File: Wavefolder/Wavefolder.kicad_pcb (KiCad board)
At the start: 2 copper layers, 25 x 200 mm, 39 parts, among them J1 Sig1, J2 EuroPower, J3 Sig2, J4 Out1, J5 Out2, J6 CV2, Q1 BC547, Q2 BC557, Q3 BC557, Q4 BC547, Q5 BC557, Q6 BC547, U1 TL074, U2 TL082, U3 TL074

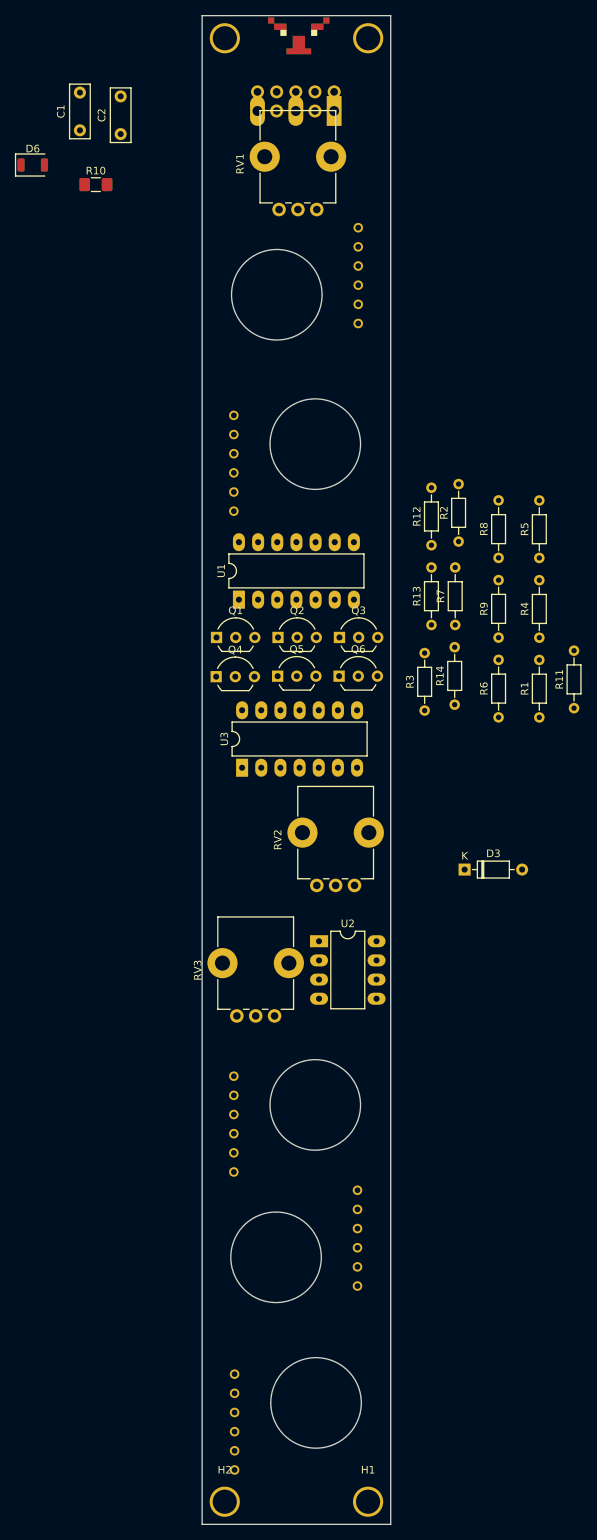
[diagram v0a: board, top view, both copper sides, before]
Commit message: Wavefolder layout
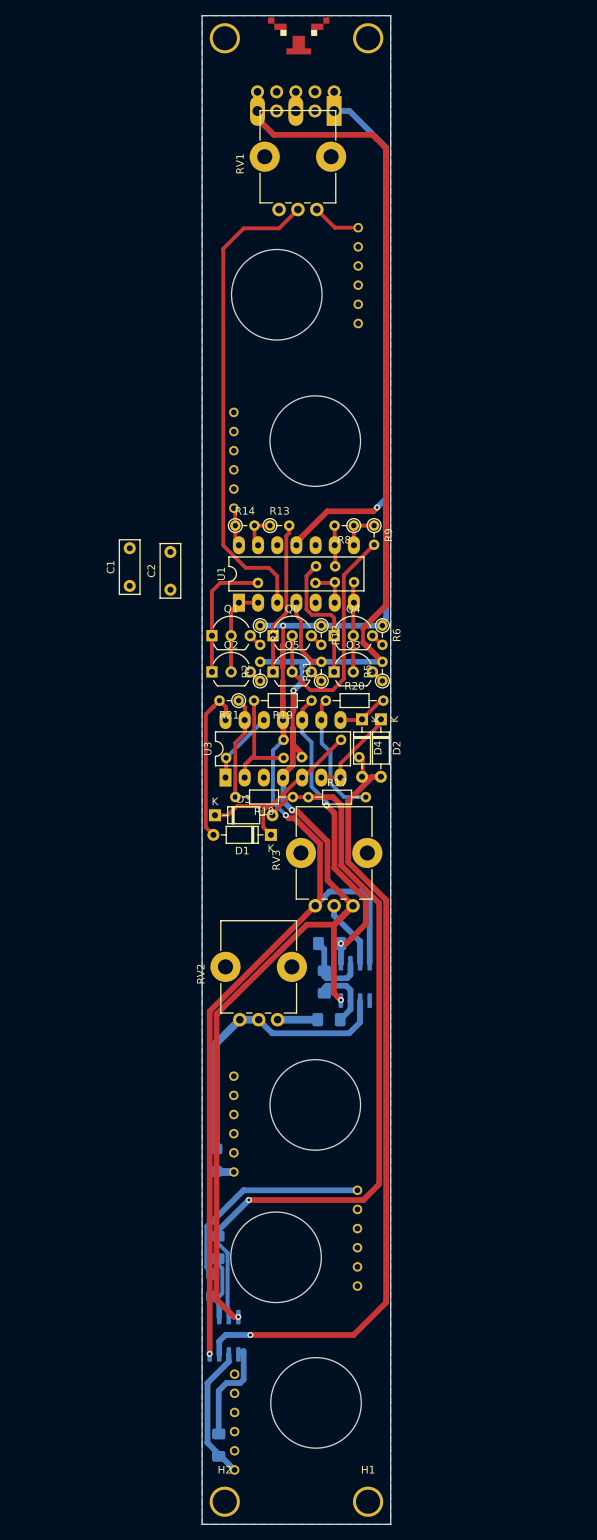
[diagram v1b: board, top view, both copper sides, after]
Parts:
- removed D6: LED, LED_SMD:LED_1206_3216Metric_ReverseMount_Hole1.8x2.4mm
- removed R10: 1k, Resistor_SMD:R_1206_3216Metric_Pad1.42x1.75mm_HandSolder
- added D1: 1N4148, Diode_THT:D_DO-35_SOD27_P7.62mm_Horizontal, F.Cu at (21.1, 120.6)
- added D2: 1N4148, Diode_THT:D_DO-35_SOD27_P7.62mm_Horizontal, F.Cu at (35.7, 105.3)
- added D4: 1N4148, Diode_THT:D_DO-35_SOD27_P7.62mm_Horizontal, F.Cu at (33.2, 105.3)
- added R15: 100k, Resistor_SMD:R_1206_3216Metric_Pad1.42x1.75mm_HandSolder, B.Cu at (13.4, 180.3)
- added R16: 100k, Resistor_SMD:R_1206_3216Metric_Pad1.42x1.75mm_HandSolder, B.Cu at (14.1, 175.3)
- added R17: 100k, Resistor_THT:R_Axial_DIN0204_L3.6mm_D1.6mm_P7.62mm_Horizontal, F.Cu at (26.1, 115.6)
- added R18: 100k, Resistor_THT:R_Axial_DIN0204_L3.6mm_D1.6mm_P7.62mm_Horizontal, F.Cu at (24.0, 115.6)
- added R19: 100k, Resistor_THT:R_Axial_DIN0204_L3.6mm_D1.6mm_P7.62mm_Horizontal, F.Cu at (26.5, 102.8)
- added R20: 100k, Resistor_THT:R_Axial_DIN0204_L3.6mm_D1.6mm_P7.62mm_Horizontal, F.Cu at (28.4, 102.8)
- added R21: 100k, Resistor_THT:R_Axial_DIN0204_L3.6mm_D1.6mm_P2.54mm_Vertical, F.Cu at (16.8, 102.8)
- added R22: 100k, Resistor_THT:R_Axial_DIN0204_L3.6mm_D1.6mm_P7.62mm_Horizontal, B.Cu at (22.8, 110.4)
- added R23: 15k, Resistor_THT:R_Axial_DIN0204_L3.6mm_D1.6mm_P7.62mm_Horizontal, B.Cu at (22.8, 108.0)
- added R24: 15k, Resistor_THT:R_Axial_DIN0204_L3.6mm_D1.6mm_P7.62mm_Horizontal, B.Cu at (32.8, 110.3)
- added R25: 1k, Resistor_SMD:R_1206_3216Metric_Pad1.42x1.75mm_HandSolder, B.Cu at (14.2, 201.5)
- added R26: 100k, Resistor_SMD:R_1206_3216Metric_Pad1.42x1.75mm_HandSolder, B.Cu at (13.8, 163.7)
- added R27: 100k, Resistor_SMD:R_1206_3216Metric_Pad1.42x1.75mm_HandSolder, B.Cu at (28.8, 145.1)
- added R28: 100k, Resistor_SMD:R_1206_3216Metric_Pad1.42x1.75mm_HandSolder, B.Cu at (28.2, 140.1)
- added R29: 100k, Resistor_SMD:R_1206_3216Metric_Pad1.42x1.75mm_HandSolder, B.Cu at (28.9, 135.0)
- added U4: TL082, Package_SO:SOIC-8_3.9x4.9mm_P1.27mm, B.Cu at (14.9, 187.0)
- R1, R11, R12, R13, R14, R2, R5, R6, R8, R9: footprint Resistor_THT:R_Axial_DIN0204_L3.6mm_D1.6mm_P7.62mm_Horizontal -> Resistor_THT:R_Axial_DIN0204_L3.6mm_D1.6mm_P2.54mm_Vertical
- R3: moved to B.Cu
- R4, R7: footprint Resistor_THT:R_Axial_DIN0204_L3.6mm_D1.6mm_P7.62mm_Horizontal -> Resistor_THT:R_Axial_DIN0204_L3.6mm_D1.6mm_P2.54mm_Vertical; moved to B.Cu
- U2: footprint Package_DIP:DIP-8_W7.62mm_LongPads -> Package_SO:SOIC-8_3.9x4.9mm_P1.27mm; moved to B.Cu
- moved C1 60.8 mm to (2.40, 87.6)
- moved C2 60.8 mm to (7.80, 88.1)
- moved R1 39.0 mm to (19.7, 92.9), turned to 270 degrees
- moved R14 37.5 mm to (16.4, 79.6), turned to 0 degrees
- moved D3 33.9 mm to (13.7, 118.0)
- moved R11 33.7 mm to (27.8, 100.2)
- moved R2 32.1 mm to (19.7, 100.2)
- moved R4 28.1 mm to (29.6, 87.1), turned to 0 degrees
- moved R3 27.8 mm to (19.4, 87.2), turned to 0 degrees
- moved R5 26.4 mm to (35.9, 100.2)
- moved R13 25.1 mm to (21.0, 79.6), turned to 0 degrees
- moved R9 22.2 mm to (34.8, 79.6), turned to 270 degrees
- moved RV2 20.5 mm to (22.0, 145.1)
- moved R7 20.0 mm to (27.1, 85.0), turned to 0 degrees
- moved R8 19.7 mm to (32.1, 79.6), turned to 180 degrees
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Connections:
- D3 pad 1: Net-(D3-Pad1) -> Net-(D1-Pad1)
- D3 pad 2: Net-(D3-Pad2) -> /~Sig2
- R13 pad 1: Net-(Q5-Pad1) -> Net-(R13-Pad1)
- R13 pad 2: Net-(R13-Pad2) -> Net-(Q5-Pad1)
- R14 pad 1: Net-(R13-Pad2) -> /Out1
- R14 pad 2: /Out1 -> Net-(R13-Pad1)
- R8 pad 1: Net-(R7-Pad2) -> Net-(R8-Pad1)
- R8 pad 2: Net-(R8-Pad2) -> Net-(R7-Pad2)
- R9 pad 1: Net-(R8-Pad2) -> Net-(R8-Pad1)
- RV2 pad 2: Net-(RV2-Pad2) -> Net-(R26-Pad2)
- RV2 pad 3: Net-(RV2-Pad3) -> Net-(R26-Pad2)
- RV3 pad 1: Net-(RV3-Pad1) -> +12V
- RV3 pad 3: Net-(RV3-Pad3) -> -12V
- U1 pad 1: (no net) -> Net-(Q1-Pad2)
- U1 pad 13: Net-(R13-Pad2) -> Net-(R13-Pad1)
- U1 pad 2: (no net) -> Net-(Q1-Pad2)
- U1 pad 3: (no net) -> Net-(RV1-Pad2)
- U1 pad 8: Net-(R8-Pad2) -> Net-(R8-Pad1)
- U2 pad 1: Net-(U2-Pad1) -> /Offset
- U2 pad 3: Net-(U2-Pad3) -> Net-(RV3-Pad2)
- U2 pad 5: Net-(U2-Pad5) -> GND
- U2 pad 6: Net-(U2-Pad6) -> Net-(R26-Pad2)
- U3 pad 1: (no net) -> /~Offset
- U3 pad 10: (no net) -> /Offset
- U3 pad 11: (no net) -> -12V
- U3 pad 12: (no net) -> /~Offset
- U3 pad 13: (no net) -> Net-(R18-Pad2)
- U3 pad 14: (no net) -> /Bottom
- U3 pad 2: (no net) -> Net-(R19-Pad2)
- U3 pad 3: (no net) -> GND
- U3 pad 4: (no net) -> +12V
- U3 pad 5: Net-(U3-Pad5) -> Net-(D1-Pad1)
- U3 pad 6: Net-(U3-Pad6) -> Net-(D2-Pad1)
- U3 pad 7: Net-(U3-Pad7) -> Net-(D2-Pad1)
- U3 pad 8: (no net) -> /Top
- U3 pad 9: (no net) -> Net-(R17-Pad2)
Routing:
- net +12V: track 0.00 -> 247.2 mm, vias 0 -> 4
- net -12V: track 0.00 -> 229.7 mm, vias 0 -> 4
- net /Out2: track 0.00 -> 105.4 mm, vias 0 -> 1
- net /~Sig2: track 0.00 -> 98.9 mm, vias 0 -> 1
- net Net-(RV1-Pad2): track 0.00 -> 63.7 mm
- net /Offset: track 0.00 -> 40.6 mm, vias 0 -> 2
- net Net-(R26-Pad2): track 0.00 -> 38.6 mm
- net Net-(Q5-Pad2): track 0.00 -> 32.7 mm
- net /Sig2: track 0.00 -> 28.5 mm
- net Net-(D1-Pad1): track 0.00 -> 25.8 mm
- net /Bottom: track 0.00 -> 23.5 mm
- net Net-(Q5-Pad1): track 0.00 -> 20.3 mm
- net Net-(J5-PadT): track 0.00 -> 18.0 mm
- net Net-(Q3-Pad1): track 0.00 -> 17.5 mm
- net Net-(Q1-Pad1): track 0.00 -> 17.3 mm
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- added copper zone on B.Cu, net GND
